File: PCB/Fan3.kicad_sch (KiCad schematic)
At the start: 5 parts, among them J3 Conn_01x02, Q3 IRLML0030

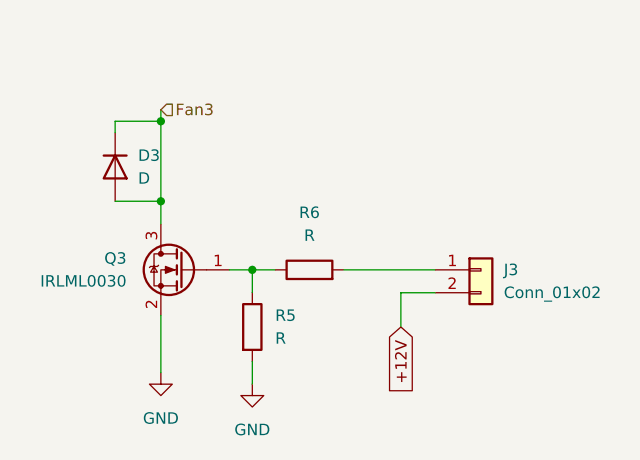
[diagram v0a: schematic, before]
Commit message: finished PCB
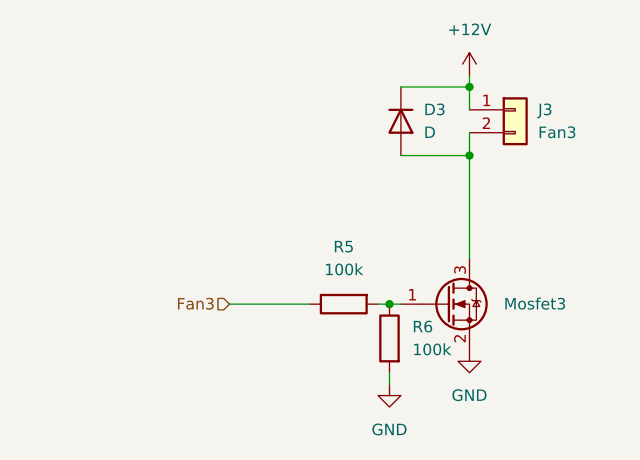
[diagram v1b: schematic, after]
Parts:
- removed Q3: IRLML0030, Package_TO_SOT_SMD:SOT-23, symbol Transistor_FET:IRLML0030
- added Mosfet3: IRLML0030, Package_TO_SOT_SMD:SOT-23, symbol Transistor_FET:IRLML0030
- J3: value Conn_01x02 -> Fan3
- R5, R6: value R -> 100k
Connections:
- net +12V: now also D3.1 (K), J3.1 (Pin_1); no longer J3.2 (Pin_2)
- net Fan3: now also R5.1; no longer D3.1 (K), D3.2 (A)
- net GND: now also R6.2, Mosfet3.2 (S); no longer R5.2
- net at R6.1: now also R5.2, Mosfet3.1 (G); no longer R5.1
- new net: D3.2 (A), J3.2 (Pin_2), Mosfet3.3 (D)
